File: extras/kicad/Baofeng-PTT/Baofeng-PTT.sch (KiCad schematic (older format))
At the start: 18 parts, among them J1 AI, J2 AO, J3 Conn_01x02_Male, J4 PTT, J5 Conn_01x02_Male, J6 Conn_01x02_Male, J7 Conn_01x02_Male, J8 Baofeng, U1 ULN2003

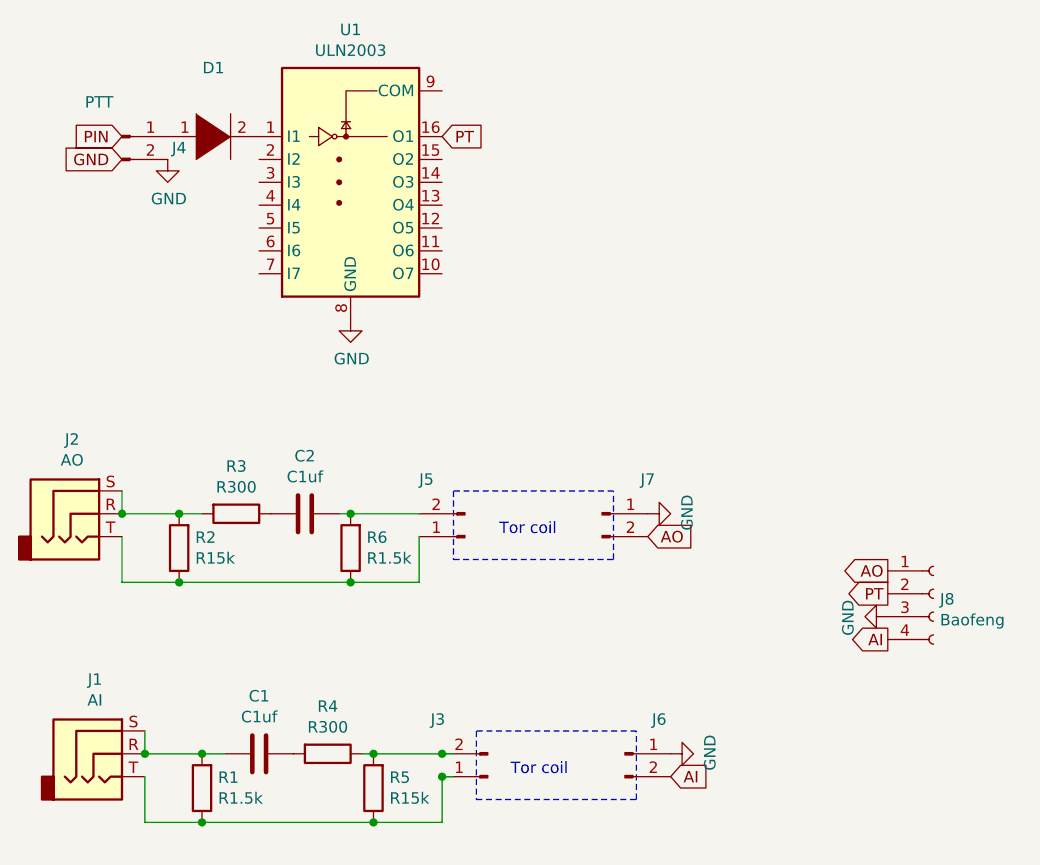
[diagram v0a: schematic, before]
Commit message: Cleanup kikad
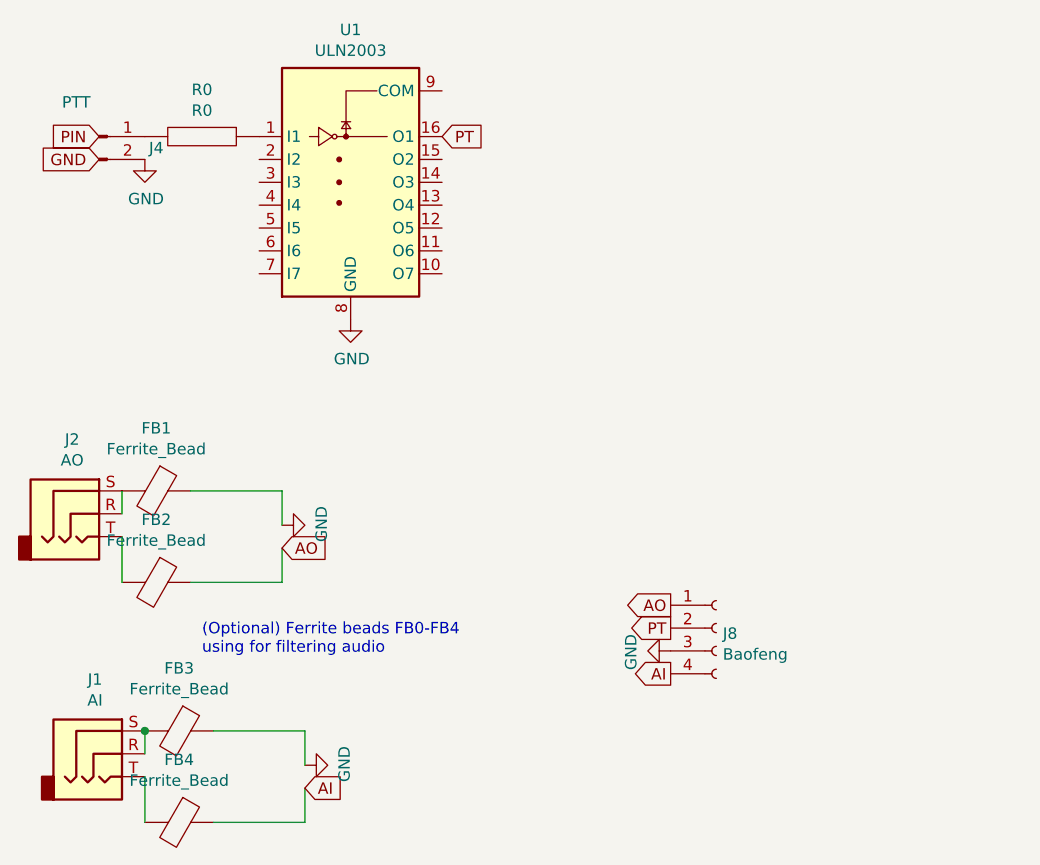
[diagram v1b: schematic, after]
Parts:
- removed C1, C2: C1uf, Capacitor_THT:C_Disc_D3.0mm_W1.6mm_P2.50mm, symbol Device:C
- removed D1: DIODE, Diode_THT:D_A-405_P7.62mm_Horizontal, symbol pspice:DIODE
- removed J3, J5, J6, J7: Conn_01x02_Male, Connector_PinHeader_2.54mm:PinHeader_1x02_P2.54mm_Vertical, symbol Connector:Conn_01x02_Male
- removed R1, R6: R1.5k, Resistor_THT:R_Axial_DIN0204_L3.6mm_D1.6mm_P2.54mm_Vertical, symbol Device:R
- removed R2, R5: R15k, Resistor_THT:R_Axial_DIN0204_L3.6mm_D1.6mm_P2.54mm_Vertical, symbol Device:R
- removed R3, R4: R300, Resistor_THT:R_Axial_DIN0204_L3.6mm_D1.6mm_P2.54mm_Vertical, symbol Device:R
- added FB1, FB2, FB3, FB4: Ferrite_Bead, Connector_PinHeader_2.54mm:PinHeader_1x02_P2.54mm_Vertical, symbol Device:Ferrite_Bead
- added R0: R0, Resistor_THT:R_Axial_DIN0207_L6.3mm_D2.5mm_P7.62mm_Horizontal, symbol pspice:R
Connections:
- wire segments 22 -> 12
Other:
- note added: "(Optional) Ferrite beads FB0-FB4\nusing for filtering audio\n\n"
- note removed: "Tor coil"
- moved on the sheet: J4, J8
